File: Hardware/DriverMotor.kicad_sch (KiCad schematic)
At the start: 0 parts

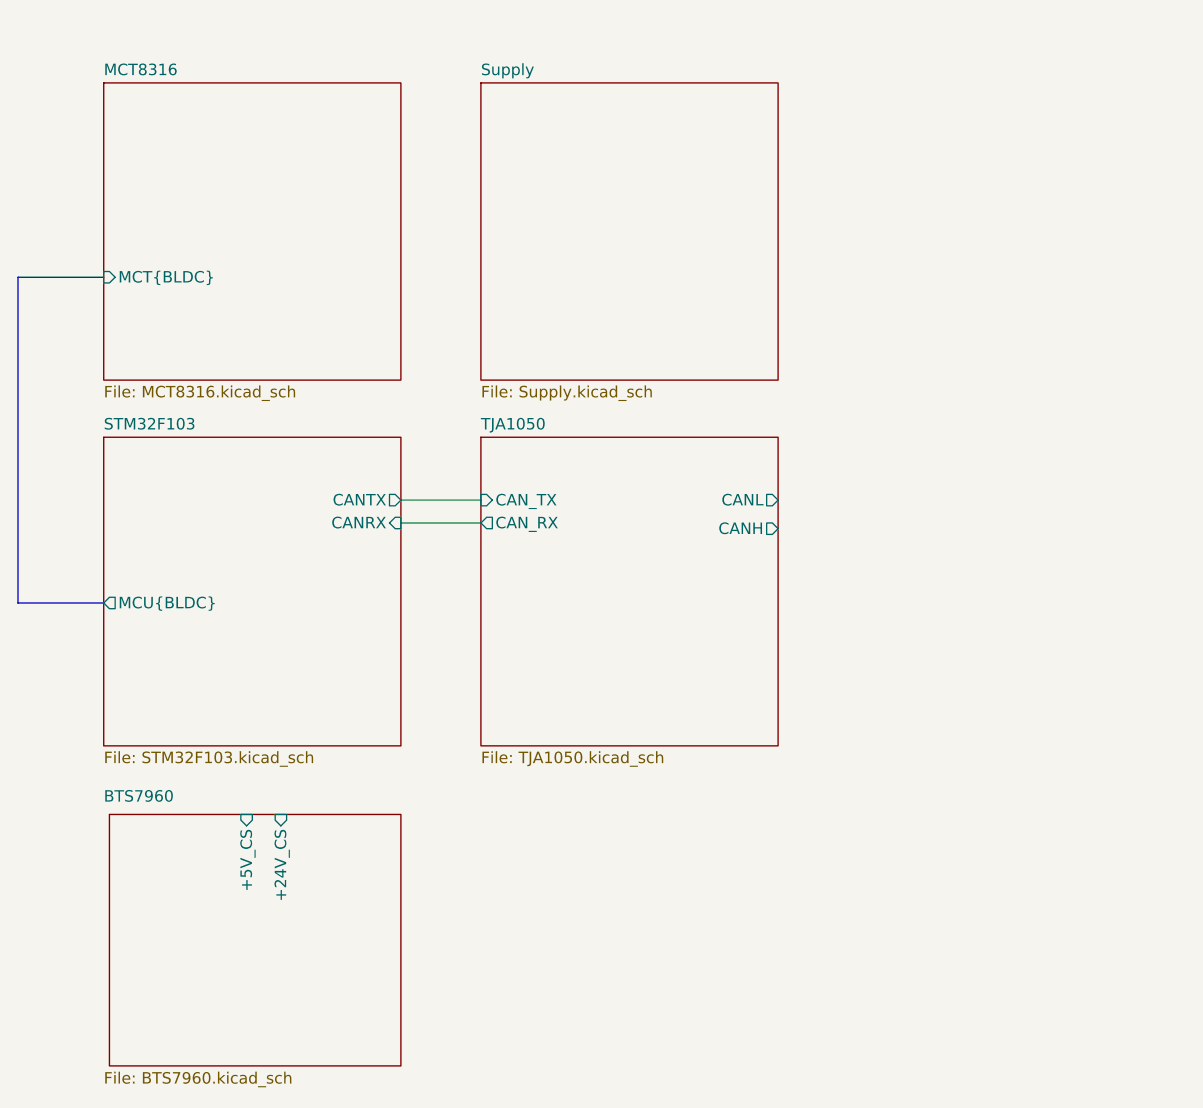
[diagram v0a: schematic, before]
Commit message: Add PCB
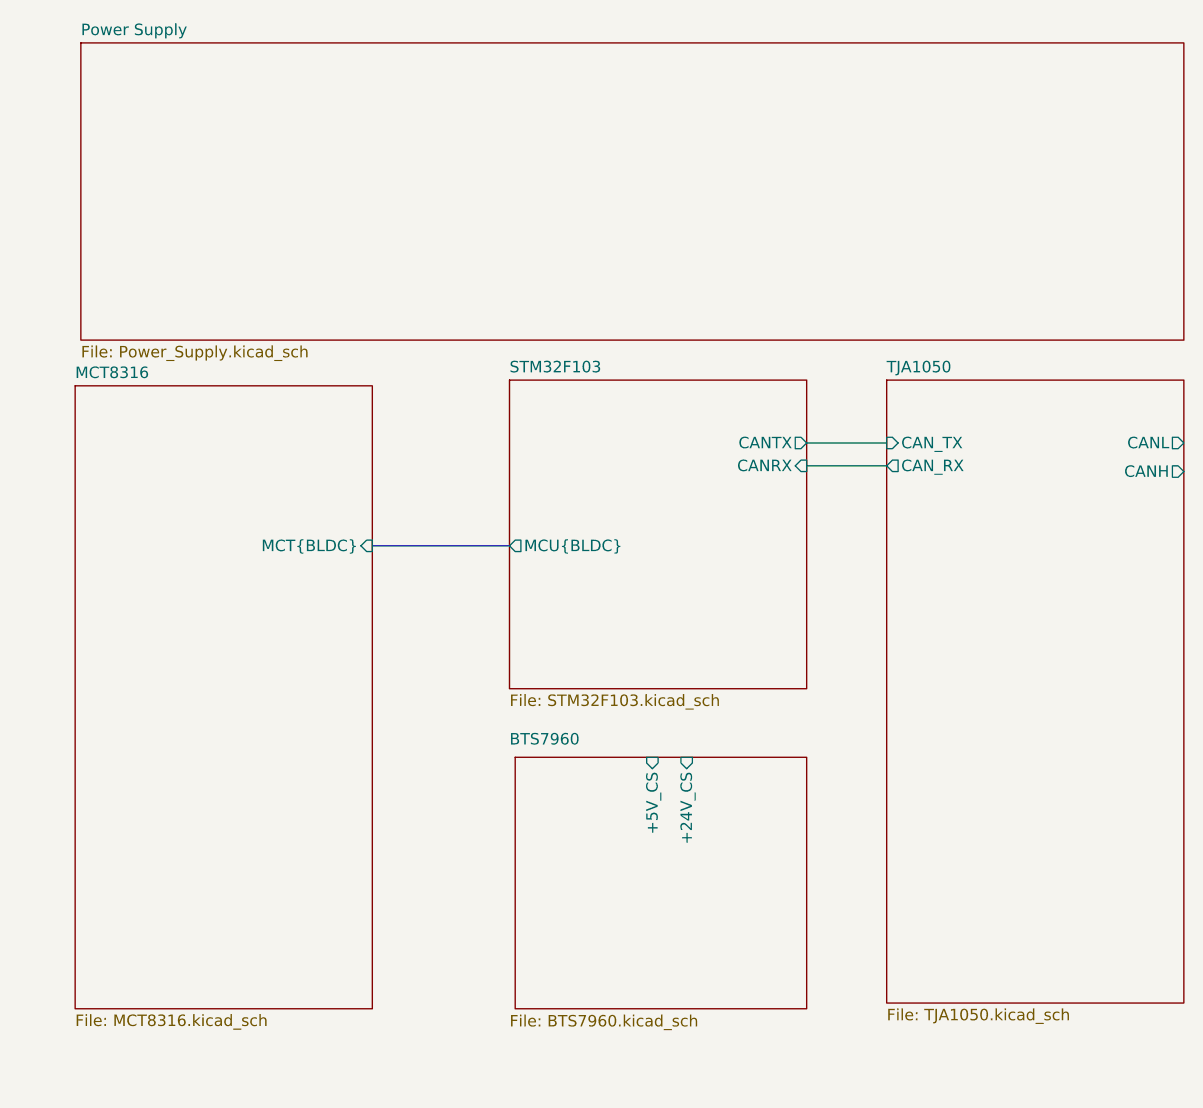
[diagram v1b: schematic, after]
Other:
- sheet Supply renamed Power Supply
- sheet Power Supply: file Supply.kicad_sch -> Power_Supply.kicad_sch
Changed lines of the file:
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@@
 (kicad_sch (version 20230121) (generator eeschema)
   (paper "A4")
-  (bus (pts (xy 73.025 92.71) (xy 82.55 92.71))
+  (bus (pts (xy 112.395 86.36) (xy 127.635 86.36))
     (stroke (width 0) (type default))
   )
-  (wire (pts (xy 115.57 83.82) (xy 124.46 83.82))
+  (wire (pts (xy 160.655 77.47) (xy 169.545 77.47))
     (stroke (width 0) (type default))
   )
-  (bus (pts (xy 73.025 56.515) (xy 73.025 92.71))
+  (wire (pts (xy 160.655 74.93) (xy 169.545 74.93))
     (stroke (width 0) (type default))
   )
-  (bus (pts (xy 82.55 56.515) (xy 73.025 56.515))
-    (stroke (width 0) (type default))
-  )
-  (wire (pts (xy 115.57 81.28) (xy 124.46 81.28))
-    (stroke (width 0) (type default))
-  )
-  (sheet (at 82.55 74.295) (size 33.02 34.29) (fields_autoplaced)
+  (sheet (at 127.635 67.945) (size 33.02 34.29) (fields_autoplaced)
     (stroke (width 0.1524) (type solid) (color 0 0 255 1))
-    (fill (color 255 255 194 1.0000))
-    (property "Sheetname" "STM32F103" (at 82.55 73.5834 0)
+    (fill (color 255 255 0 1.0000))
+    (property "Sheetname" "STM32F103" (at 127.635 67.2334 0)
       (effects (font (size 1.27 1.27)) (justify left bottom))
     )
-    (property "Sheetfile" "STM32F103.kicad_sch" (at 82.55 109.1696 0)
+    (property "Sheetfile" "STM32F103.kicad_sch" (at 127.635 102.8196 0)
       (effects (font (size 1.27 1.27)) (justify left top))
     )
-    (pin "CANTX" output (at 115.57 81.28 0)
+    (pin "CANTX" output (at 160.655 74.93 0)
       (effects (font (size 1.27 1.27)) (justify right))
     )
-    (pin "CANRX" input (at 115.57 83.82 0)
+    (pin "CANRX" input (at 160.655 77.47 0)
       (effects (font (size 1.27 1.27)) (justify right))
     )
-    (pin "MCU{BLDC}" output (at 82.55 92.71 180)
+    (pin "MCU{BLDC}" output (at 127.635 86.36 180)
       (effects (font (size 1.27 1.27)) (justify left))
     )
@@
     )
   )
-  (sheet (at 83.185 116.205) (size 32.385 27.94)
+  (sheet (at 128.27 109.855) (size 32.385 27.94)
     (stroke (width 0.1524) (type solid) (color 0 0 255 1))
-    (fill (color 255 255 194 1.0000))
-    (property "Sheetname" "BTS7960" (at 82.55 114.935 0)
+    (fill (color 255 0 0 1.0000))
+    (property "Sheetname" "BTS7960" (at 127.635 108.585 0)
       (effects (font (size 1.27 1.27)) (justify left bottom))
     )
-    (property "Sheetfile" "BTS7960.kicad_sch" (at 82.55 144.78 0)
+    (property "Sheetfile" "BTS7960.kicad_sch" (at 127.635 138.43 0)
       (effects (font (size 1.27 1.27)) (justify left top))
     )
-    (pin "+5V_CS" input (at 98.425 116.205 90)
+    (pin "+5V_CS" input (at 143.51 109.855 90)
       (effects (font (size 1.27 1.27)) (justify right))
     )
-    (pin "+24V_CS" input (at 102.235 116.205 90)
+    (pin "+24V_CS" input (at 147.32 109.855 90)
       (effects (font (size 1.27 1.27)) (justify right))
     )
@@
     )
   )
-  (sheet (at 82.55 34.925) (size 33.02 33.02) (fields_autoplaced)
+  (sheet (at 79.375 68.58) (size 33.02 69.215) (fields_autoplaced)
     (stroke (width 0.1524) (type solid) (color 0 0 255 1))
-    (fill (color 255 255 194 1.0000))
-    (property "Sheetname" "MCT8316" (at 82.55 34.2134 0)
+    (fill (color 255 0 0 1.0000))
+    (property "Sheetname" "MCT8316" (at 79.375 67.8684 0)
       (effects (font (size 1.27 1.27)) (justify left bottom))
     )
-    (property "Sheetfile" "MCT8316.kicad_sch" (at 82.55 68.5296 0)
+    (property "Sheetfile" "MCT8316.kicad_sch" (at 79.375 138.3796 0)
       (effects (font (size 1.27 1.27)) (justify left top))
     )
-    (pin "MCT{BLDC}" input (at 82.55 56.515 180)
-      (effects (font (size 1.27 1.27)) (justify left))
+    (pin "MCT{BLDC}" input (at 112.395 86.36 0)
+      (effects (font (size 1.27 1.27)) (justify right))
     )
     (instances
@@
     )
   )
-  (sheet (at 124.46 34.925) (size 33.02 33.02) (fields_autoplaced)
+  (sheet (at 80.01 30.48) (size 122.555 33.02) (fields_autoplaced)
     (stroke (width 0.1524) (type solid) (color 0 0 255 1))
-    (fill (color 255 255 194 1.0000))
-    (property "Sheetname" "Supply" (at 124.46 34.2134 0)
+    (fill (color 255 0 0 1.0000))
+    (property "Sheetname" "Power Supply" (at 80.01 29.7684 0)
       (effects (font (size 1.27 1.27)) (justify left bottom))
     )
-    (property "Sheetfile" "Supply.kicad_sch" (at 124.46 68.5296 0)
+    (property "Sheetfile" "Power_Supply.kicad_sch" (at 80.01 64.0846 0)
       (effects (font (size 1.27 1.27)) (justify left top))
     )
-    (property "Field2" "" (at 124.46 34.925 0)
+    (property "Field2" "" (at 80.01 30.48 0)
       (effects (font (size 1.27 1.27)) hide)
     )
@@
     )
   )
-  (sheet (at 124.46 74.295) (size 33.02 34.29) (fields_autoplaced)
+  (sheet (at 169.545 67.945) (size 33.02 69.215) (fields_autoplaced)
     (stroke (width 0.1524) (type solid) (color 0 0 255 1))
-    (fill (color 255 255 194 1.0000))
-    (property "Sheetname" "TJA1050" (at 124.46 73.5834 0)
+    (fill (color 255 0 0 1.0000))
+    (property "Sheetname" "TJA1050" (at 169.545 67.2334 0)
       (effects (font (size 1.27 1.27)) (justify left bottom))
     )
-    (property "Sheetfile" "TJA1050.kicad_sch" (at 124.46 109.1696 0)
+    (property "Sheetfile" "TJA1050.kicad_sch" (at 169.545 137.7446 0)
       (effects (font (size 1.27 1.27)) (justify left top))
     )
-    (property "Field2" "" (at 124.46 74.295 0)
+    (property "Field2" "" (at 169.545 67.945 0)
       (effects (font (size 1.27 1.27)) hide)
     )
-    (property "Field3" "" (at 124.46 74.295 0)
+    (property "Field3" "" (at 169.545 67.945 0)
       (effects (font (size 1.27 1.27)) hide)
     )
-    (pin "CAN_TX" input (at 124.46 81.28 180)
+    (pin "CAN_TX" input (at 169.545 74.93 180)
       (effects (font (size 1.27 1.27)) (justify left))
     )
-    (pin "CAN_RX" output (at 124.46 83.82 180)
+    (pin "CAN_RX" output (at 169.545 77.47 180)
       (effects (font (size 1.27 1.27)) (justify left))
     )
-    (pin "CANL" output (at 157.48 81.28 0)
+    (pin "CANL" output (at 202.565 74.93 0)
       (effects (font (size 1.27 1.27)) (justify right))
     )
-    (pin "CANH" output (at 157.48 84.455 0)
+    (pin "CANH" output (at 202.565 78.105 0)
       (effects (font (size 1.27 1.27)) (justify right))
     )
